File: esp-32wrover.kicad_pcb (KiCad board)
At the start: 2 copper layers, 68.6 x 53.3 mm, 79 parts, among them CON1 BARREL_JACK, P1 Power, P10 ICSP, P2 Analog, P3 Digital, P4 Digital, P5 CONN_1, P6 CONN_1, P7 CONN_1, P8 CONN_1, P9 CONN_01X04, Q3 Q_NPN_BEC, Q4 Q_NPN_BEC, SW1 SW_PUSH, SW2 SW_PUSH, U1 usb_mini_b, U2 MCP16311-MNY, U3 BD00GA5WEFJ, U4 PL2303HXA, U5 MCP6001R, U6 ESP32-WROVER, U7 IRLM6402, Y1 12Mhz, Y2 32.768Khz

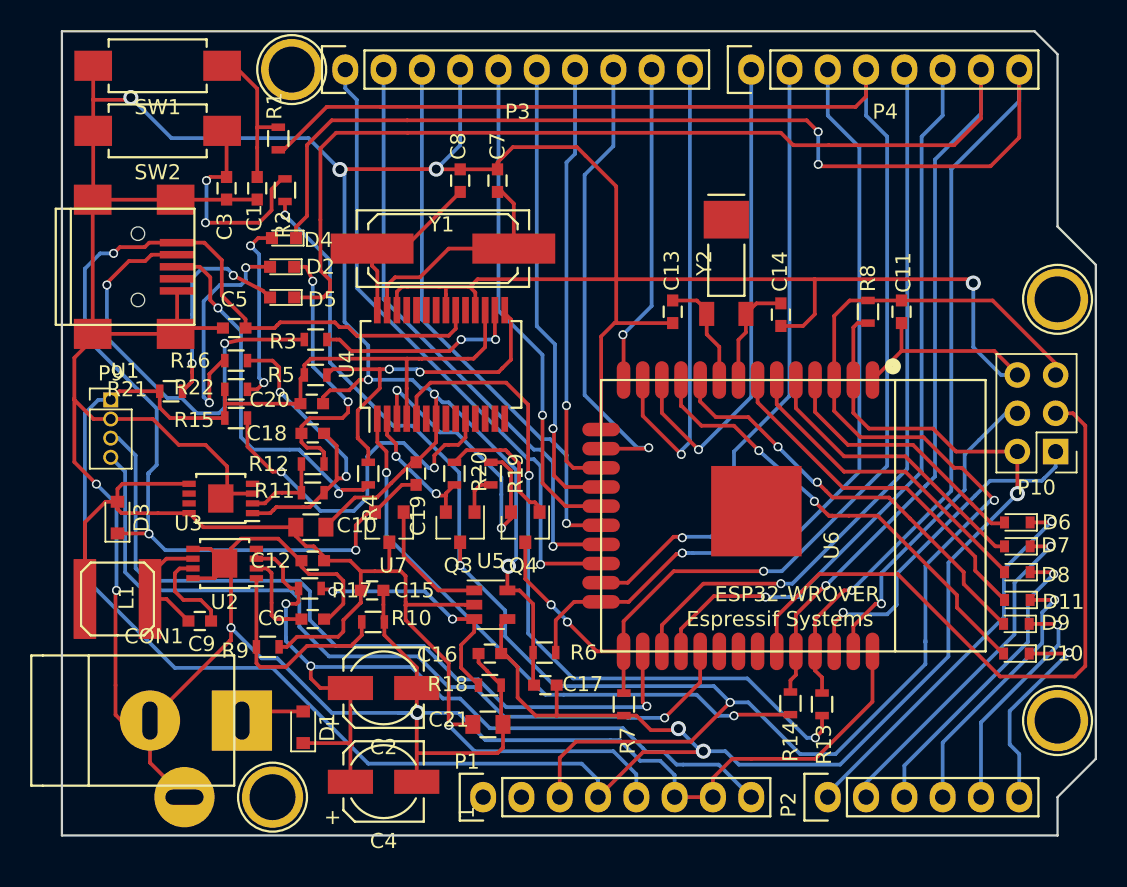
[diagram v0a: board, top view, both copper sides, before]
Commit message: xoá file autosave
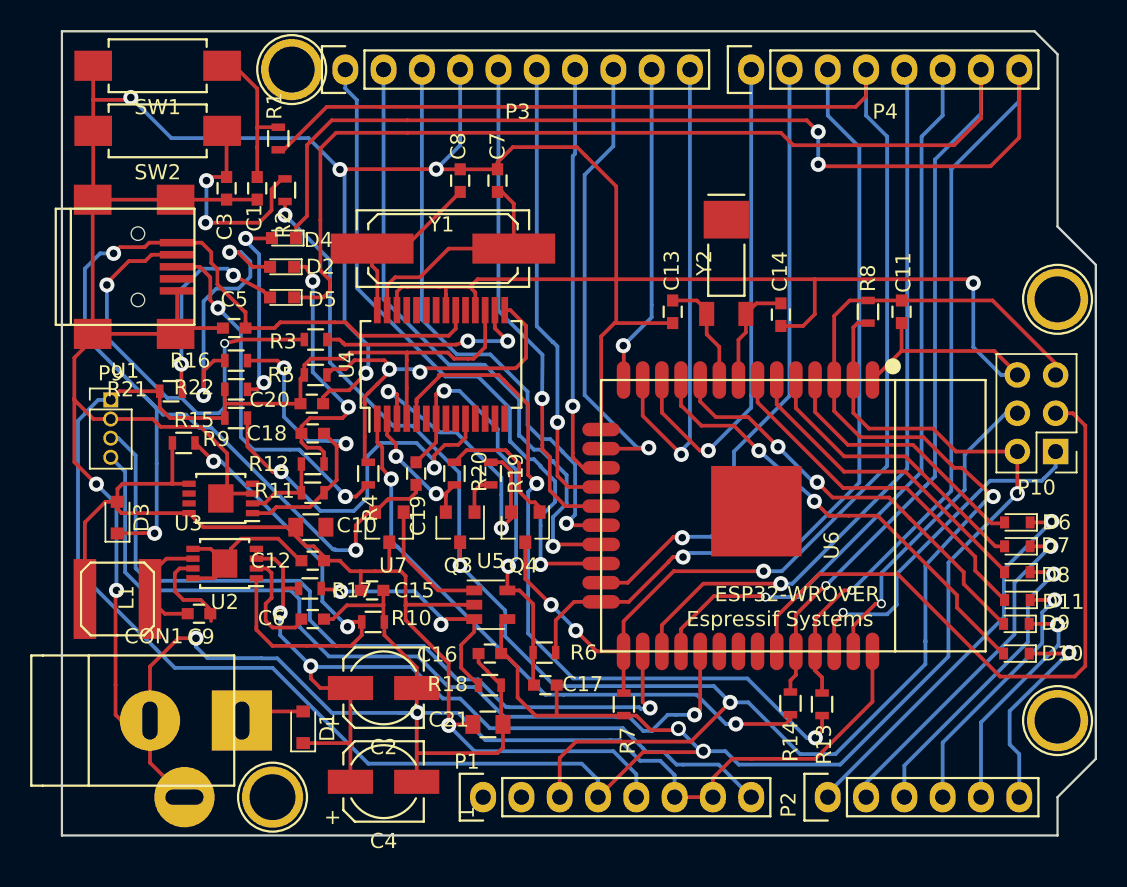
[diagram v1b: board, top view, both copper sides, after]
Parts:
- moved R9 14.6 mm to (119.1, 100.3), turned to 0 degrees
- moved C9 0.49 mm to (120.1, 111.7)
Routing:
- net GND: track 406.1 -> 390.4 mm
- net Net-(R10-Pad1): track 14.8 -> 30.1 mm, vias 0 -> 2
- net +5V: track 79.6 -> 74.5 mm
- net VCC: track 74.2 -> 78.8 mm
- net Net-(D2-Pad2): track 16.0 -> 19.4 mm
- net SDO: track 39.8 -> 42.2 mm
- net Net-(R4-Pad1): track 23.4 -> 25.6 mm
- net SD1: track 42.5 -> 44.6 mm
- net SDA: track 54.3 -> 56.1 mm
- net CLK: track 37.0 -> 38.5 mm
- net Net-(C6-Pad1): track 6.01 -> 7.34 mm
- net +3V3: track 175.5 -> 176.6 mm
- net Net-(R13-Pad1): track 48.7 -> 49.5 mm
- net Net-(R3-Pad1): track 13.8 -> 14.6 mm
- net SD2: track 28.7 -> 28.0 mm
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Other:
- net class Default: via_drill 0.6 -> 0.5
